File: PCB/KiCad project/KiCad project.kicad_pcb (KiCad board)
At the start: 2 copper layers, 69.1 x 74.3 mm, 7 parts, among them SW2 SW_Push, SW3 SW_Push, SW4 SW_Push, U1 XIAO-RP2040-DIP, U2 OLED_0.91_128x32

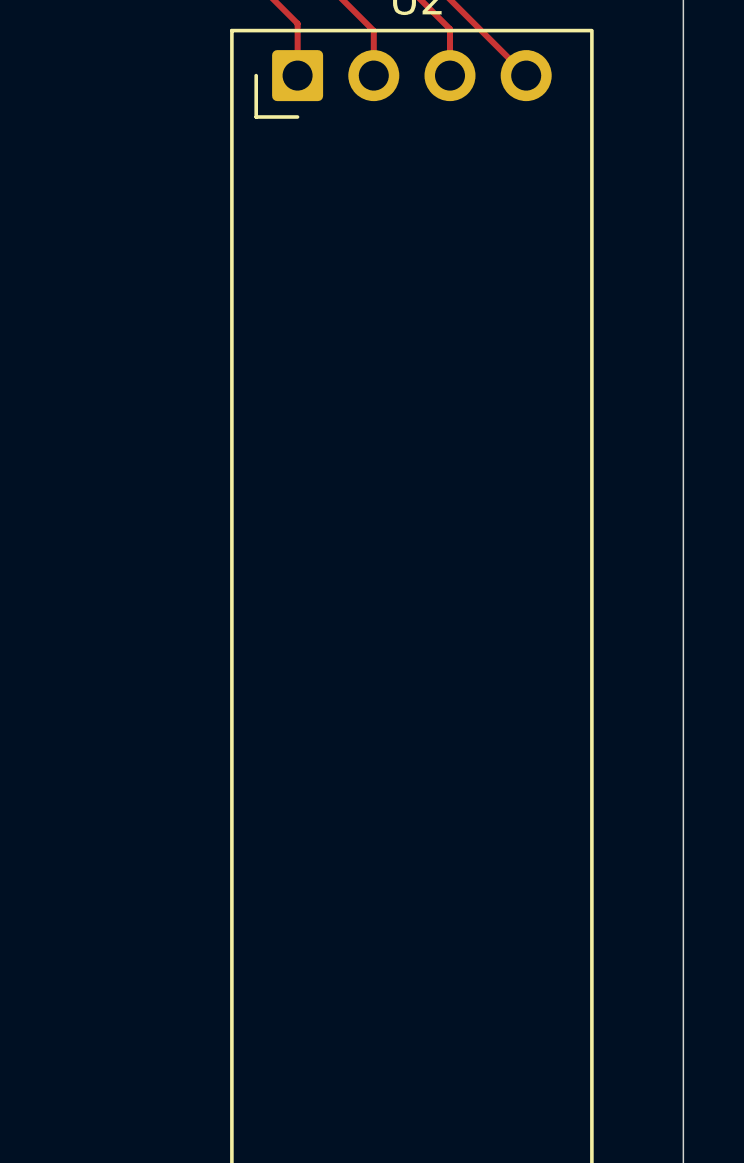
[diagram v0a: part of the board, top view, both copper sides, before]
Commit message: Add files via upload
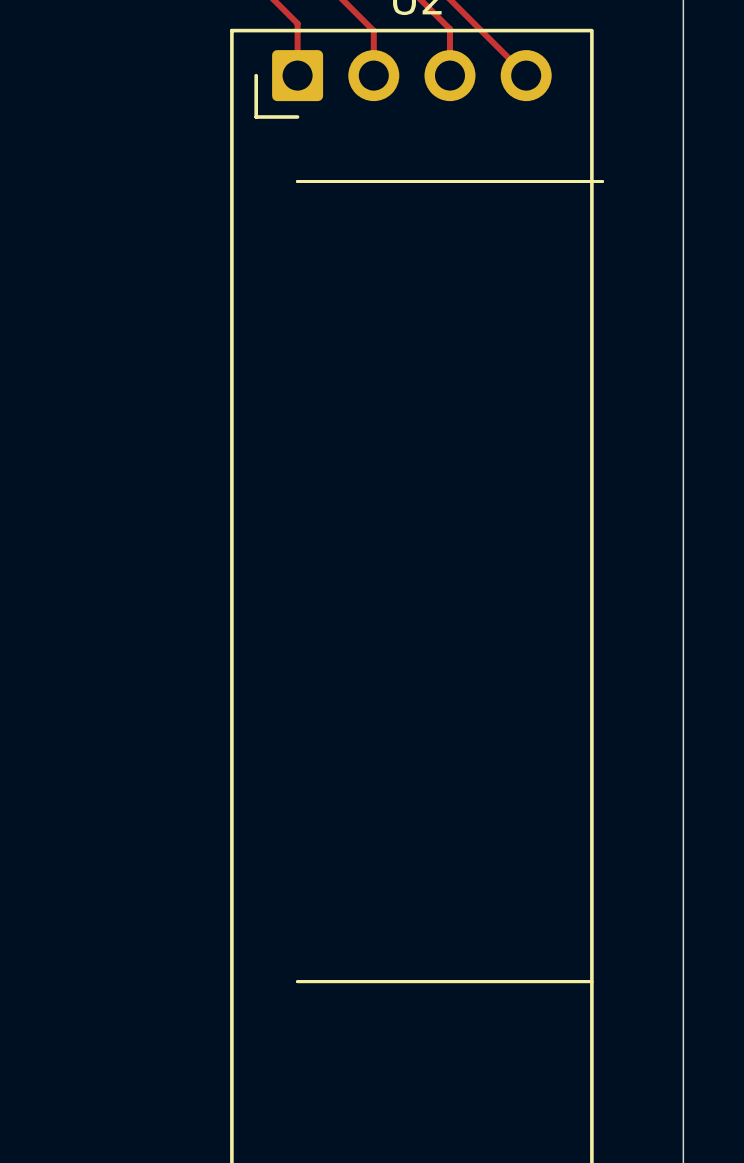
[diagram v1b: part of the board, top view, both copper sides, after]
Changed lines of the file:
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@@
+	)
+	(gr_rect
+		(start 175.26 90.17)
+		(end 185.07 90.17)
+		(stroke
+			(width 0.1)
+			(type default)
+		)
+		(fill no)
+		(layer "F.SilkS")
+	)
+	(gr_rect
+		(start 175.26 63.5)
+		(end 185.42 63.5)
+		(stroke
+			(width 0.1)
+			(type default)
+		)
+		(fill no)
+		(layer "F.SilkS")
 	)
 	(gr_rect
